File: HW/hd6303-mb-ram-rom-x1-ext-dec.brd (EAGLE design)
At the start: 100 x 80 mm, 37 parts, among them IC1 74HC138N, IC2 AM29F010N

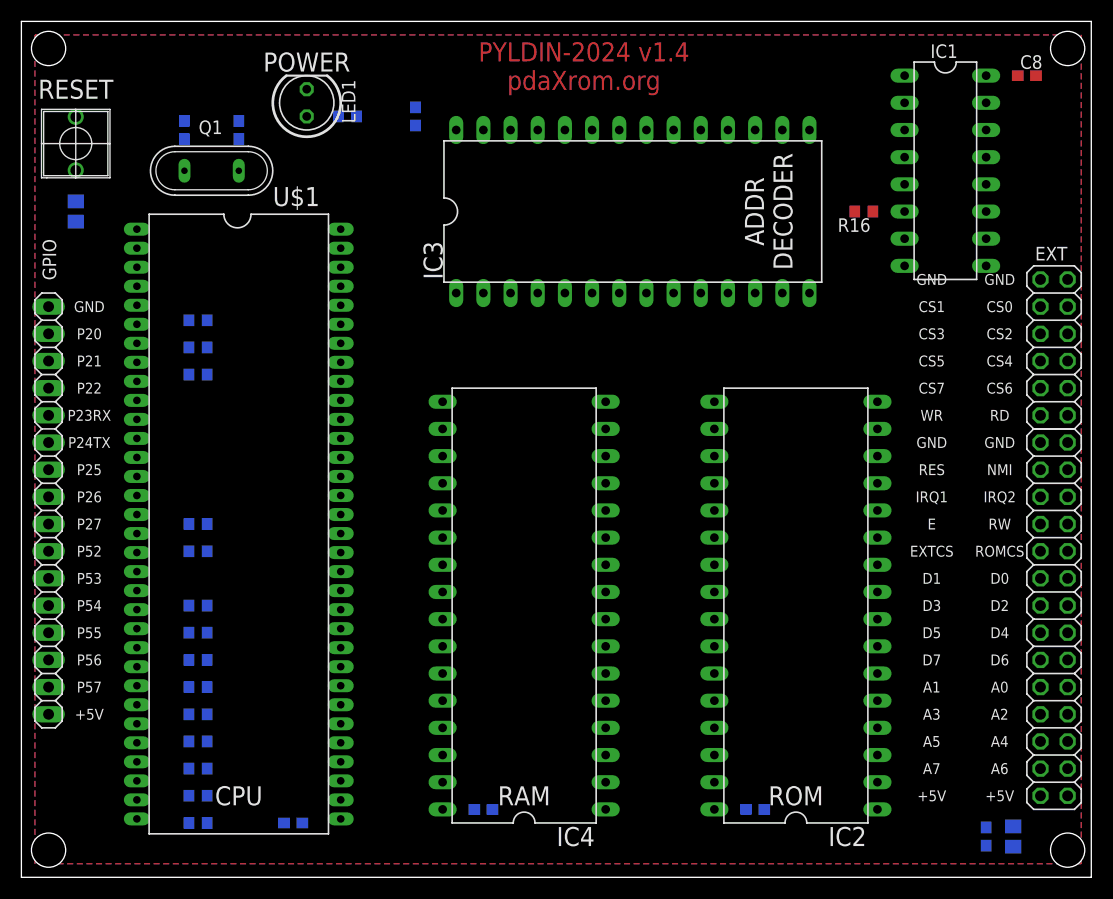
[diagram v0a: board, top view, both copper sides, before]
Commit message: traced pcb
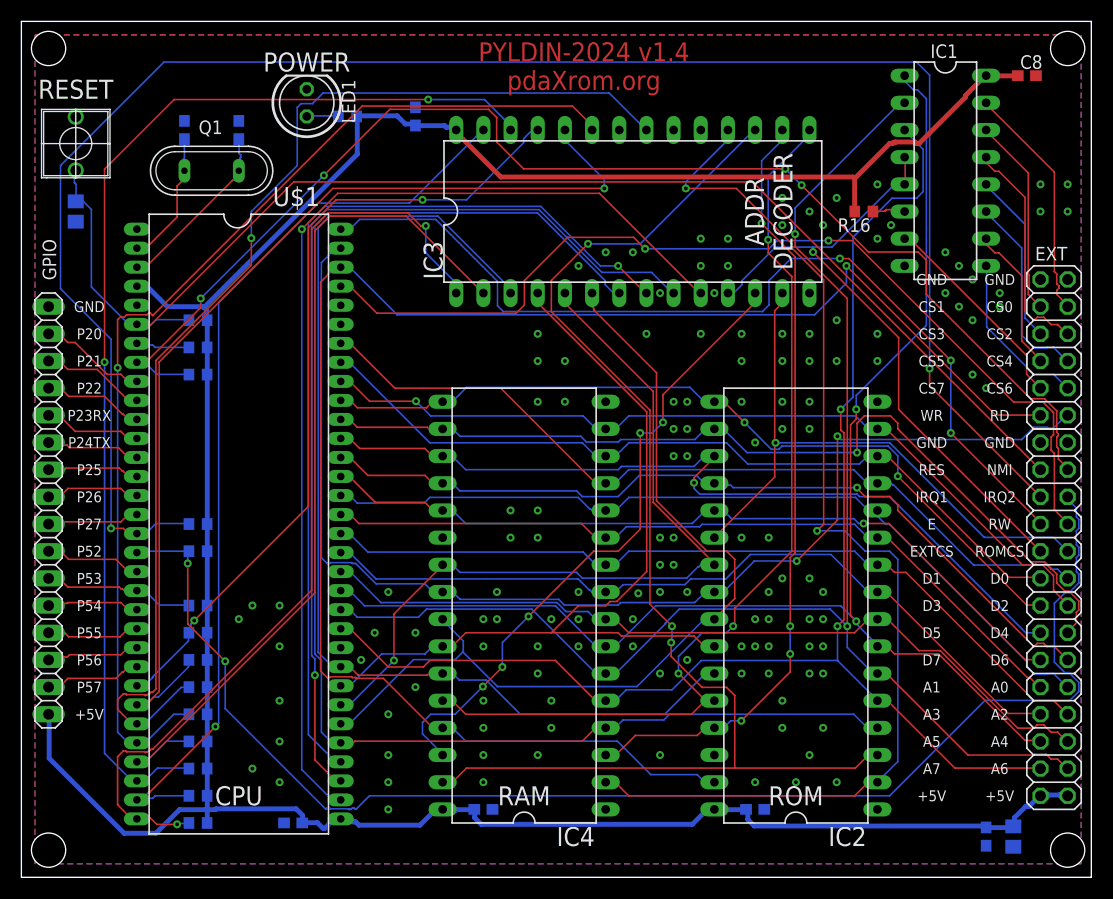
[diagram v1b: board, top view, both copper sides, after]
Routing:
- net +5V: track 0.00 -> 261.2 mm
- net IRQ1: track 0.00 -> 173.2 mm, vias 0 -> 2
- net WR: track 0.00 -> 155.9 mm, vias 0 -> 1
- net A6: track 0.00 -> 136.4 mm, vias 0 -> 2
- net A12: track 0.00 -> 133.9 mm
- net IRQ2: track 0.00 -> 130.9 mm, vias 0 -> 2
- net A5: track 0.00 -> 129.9 mm, vias 0 -> 2
- net A7: track 0.00 -> 129.7 mm, vias 0 -> 2
- net RES: track 0.00 -> 124.1 mm
- net NMI: track 0.00 -> 122.6 mm, vias 0 -> 4
- net MEM_A15: track 0.00 -> 120.7 mm, vias 0 -> 3
- net RD: track 0.00 -> 113.9 mm, vias 0 -> 2
- net PAGE_A15: track 0.00 -> 108.1 mm, vias 0 -> 1
- net PAGE_FN1: track 0.00 -> 106.1 mm, vias 0 -> 2
- net MEM_A16: track 0.00 -> 104.2 mm, vias 0 -> 2
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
